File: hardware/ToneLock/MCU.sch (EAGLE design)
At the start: 47 parts, among them Q1 IRLML6346, U1 LD1117S33TR, U2 MP45DT02, U3 LIS3DSHTR, X3 MINI-USB-32005-201

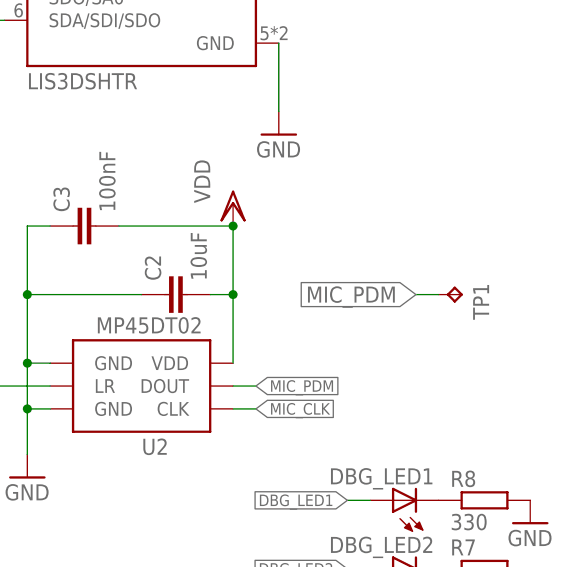
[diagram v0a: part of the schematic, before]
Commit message: Hardware ready to generate gerber
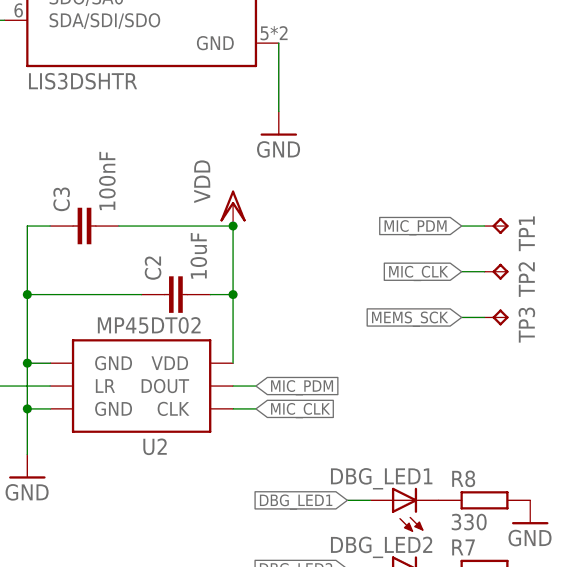
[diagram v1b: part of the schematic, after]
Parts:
- added TP2, TP3: TPB2,54, testpad:TPB2,54
- TP1: value TPB1,27 -> TPB2,54; device testpad:TPB1,27 -> testpad:TPB2,54
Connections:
- net MEMS_SCK: now also TP3.TP
- net MIC_CLK: now also TP2.TP
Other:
- moved on the sheet: TP1
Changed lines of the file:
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@@
 <part name="P+5" library="supply1" library_urn="urn:adsk.eagle:library:371" deviceset="+12V" device=""/>
 <part name="C17" library="resistor" library_urn="urn:adsk.eagle:library:348" deviceset="C-EU" device="C0603" package3d_urn="urn:adsk.eagle:package:23616/2" value="100nF"/>
-<part name="TP1" library="testpad" library_urn="urn:adsk.eagle:library:385" deviceset="TP" device="B1,27" package3d_urn="urn:adsk.eagle:package:27944/1" value="TPB1,27"/>
+<part name="TP1" library="testpad" library_urn="urn:adsk.eagle:library:385" deviceset="TP" device="B2,54" package3d_urn="urn:adsk.eagle:package:27948/1" value="TPB2,54"/>
+<part name="TP2" library="testpad" library_urn="urn:adsk.eagle:library:385" deviceset="TP" device="B2,54" package3d_urn="urn:adsk.eagle:package:27948/1"/>
+<part name="TP3" library="testpad" library_urn="urn:adsk.eagle:library:385" deviceset="TP" device="B2,54" package3d_urn="urn:adsk.eagle:package:27948/1"/>
 </parts>
 <sheets>
@@
 </instance>
 <instance part="C17" gate="G$1" x="-68.58" y="134.62"/>
-<instance part="TP1" gate="G$1" x="144.78" y="96.52" rot="R270"/>
+<instance part="TP1" gate="G$1" x="149.86" y="104.14" rot="R270"/>
+<instance part="TP2" gate="G$1" x="149.86" y="99.06" rot="R270"/>
+<instance part="TP3" gate="G$1" x="149.86" y="93.98" rot="R270"/>
 </instances>
 <busses>
@@
 <label x="91.44" y="132.08" size="1.27" layer="95" rot="R180" xref="yes"/>
 </segment>
+<segment>
+<pinref part="TP3" gate="G$1" pin="TP"/>
+<wire x1="147.32" y1="93.98" x2="144.78" y2="93.98" width="0.1524" layer="91"/>
+<label x="144.78" y="93.98" size="1.27" layer="95" rot="R180" xref="yes"/>
+</segment>
 </net>
 <net name="MEMS_MOSI" class="0">
@@
 <segment>
 <pinref part="TP1" gate="G$1" pin="TP"/>
-<wire x1="142.24" y1="96.52" x2="139.7" y2="96.52" width="0.1524" layer="91"/>
-<label x="139.7" y="96.52" size="1.778" layer="95" rot="R180" xref="yes"/>
+<wire x1="147.32" y1="104.14" x2="144.78" y2="104.14" width="0.1524" layer="91"/>
+<label x="144.78" y="104.14" size="1.27" layer="95" rot="R180" xref="yes"/>
 </segment>
 </net>
@@
 <label x="121.92" y="83.82" size="1.27" layer="95" xref="yes"/>
 </segment>
-</net>
+<segment>
+<pinref part="TP2" gate="G$1" pin="TP"/>
+<wire x1="147.32" y1="99.06" x2="144.78" y2="99.06" width="0.1524" layer="91"/>
+<label x="144.78" y="99.06" size="1.27" layer="95" rot="R180" xref="yes"/>
+</segment>
+</net>
